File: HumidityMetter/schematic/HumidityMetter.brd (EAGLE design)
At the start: 100 x 68 mm, 65 parts, among them IC1 LM317, IC2 LM317, IC3 STM32F103C8T6, IC4 AM2320, J1 0, J2 0, J3 0, J4 0, K1 POWER_ON, T1 BSS84, T2 BC847, X1 +9V, X2 GND, X3 ISP

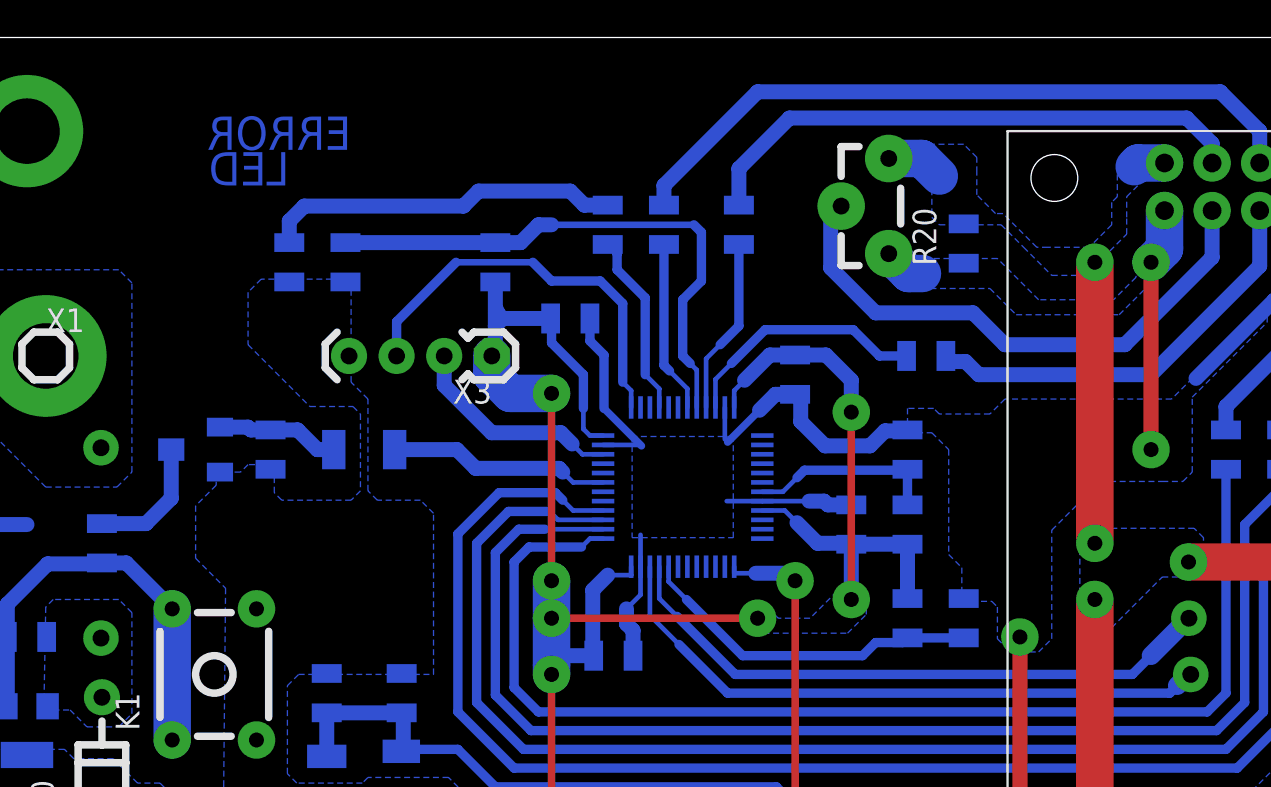
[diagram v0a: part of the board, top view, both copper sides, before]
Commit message: Himidity metter. Board routed.
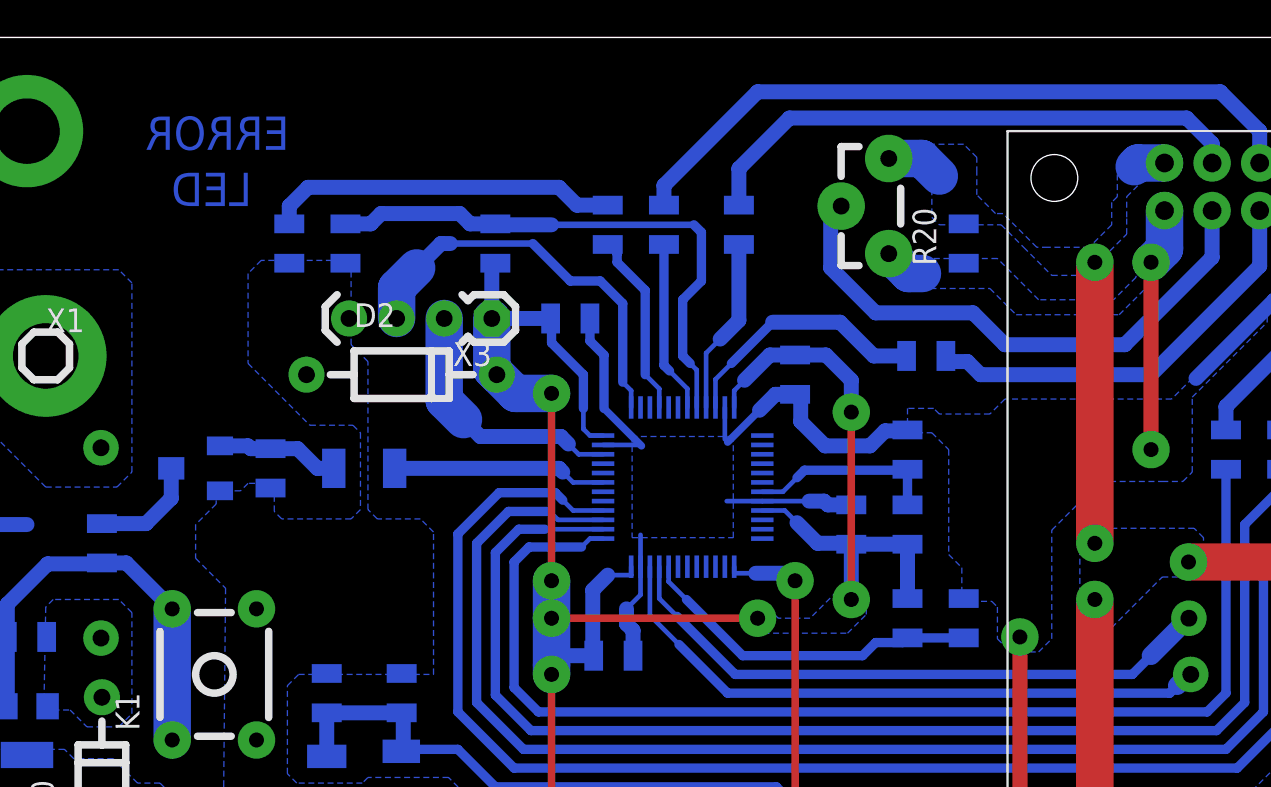
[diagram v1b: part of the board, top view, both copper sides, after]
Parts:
- added D2: 1N4007, __MyCommonLib1:DO-41_10MM
- moved X3 2.00 mm to (22.0, 48.0)
- moved J1 1.00 mm to (26.0, 52.0)
- moved J2 1.00 mm to (18.0, 52.0)
- moved LED1 1.00 mm to (15.0, 52.0)
- moved R11 1.00 mm to (19.0, 40.0)
- moved R4 1.00 mm to (14.0, 40.0)
- moved T2 1.00 mm to (10.0, 40.0)
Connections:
- net +3.3V: now also D2.CATHODE
- net GND: now also D2.ANODE
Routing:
- net SWDIO: track 11.6 -> 14.0 mm
- net N$4: track 6.86 -> 5.86 mm
